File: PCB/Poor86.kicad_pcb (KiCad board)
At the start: 4 copper layers, 100 x 170 mm, 98 parts, among them J1 Bus_ISA_8bit, J2 7-5530843-0, J3 ATX-20, P1 USB_C_Plug_USB2.0, SW3 SW_Push_Dual, SW4 SW_Push_Dual, U1 LFE5U-25F-6BG256C, U10 IS66WVE4M16EBLL-70BLI, U11 CH552T, U2 TLV62569DBV, U3 AM5x86 PQFP208, U4 TLV62569DBV, U5 ESP-12F, U6 TLV62569DBV, U9 IS66WVE4M16EBLL-70BLI

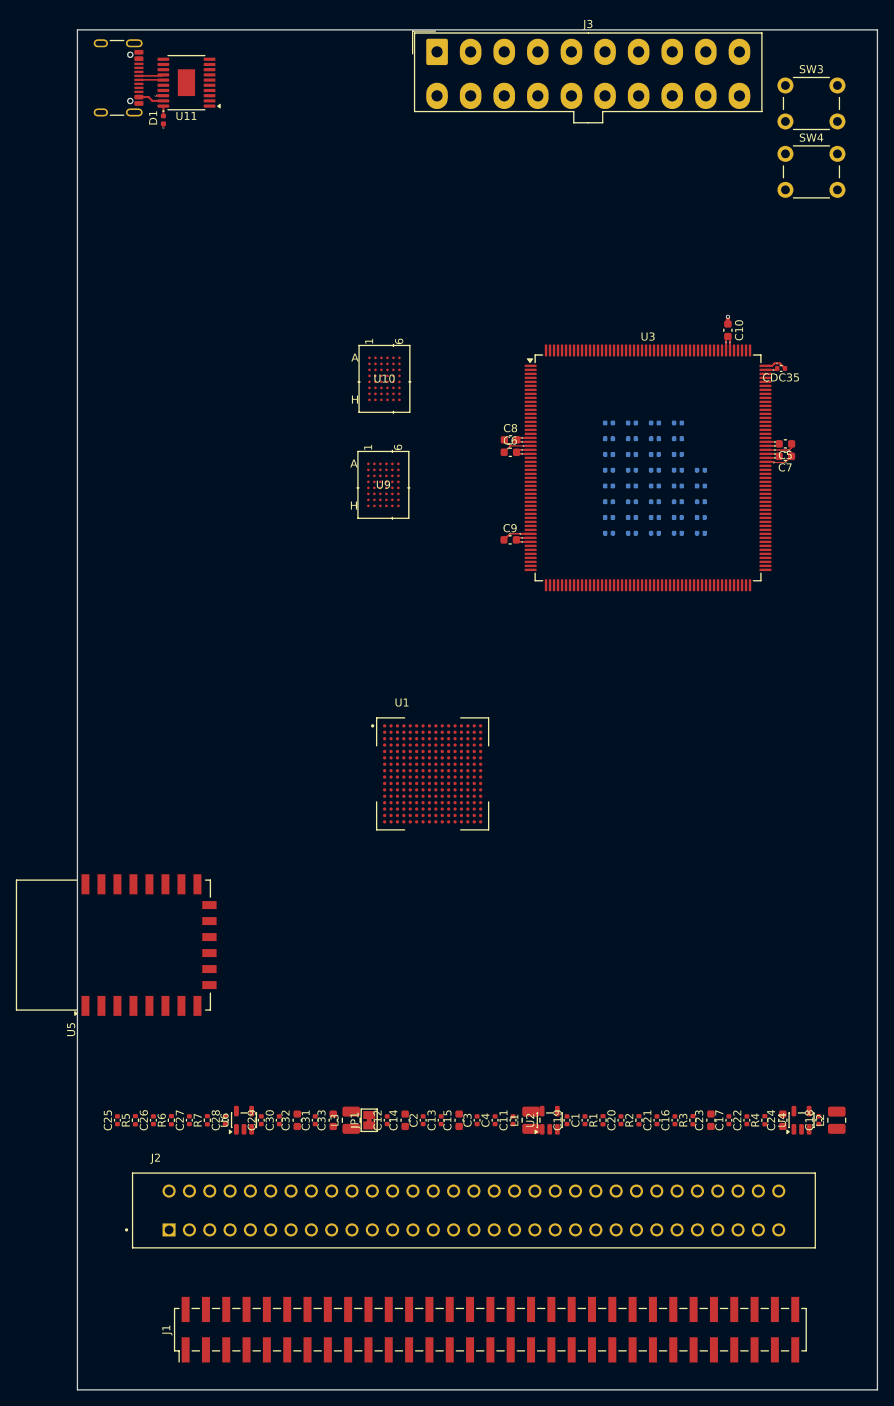
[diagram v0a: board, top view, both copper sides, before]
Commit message: more progress
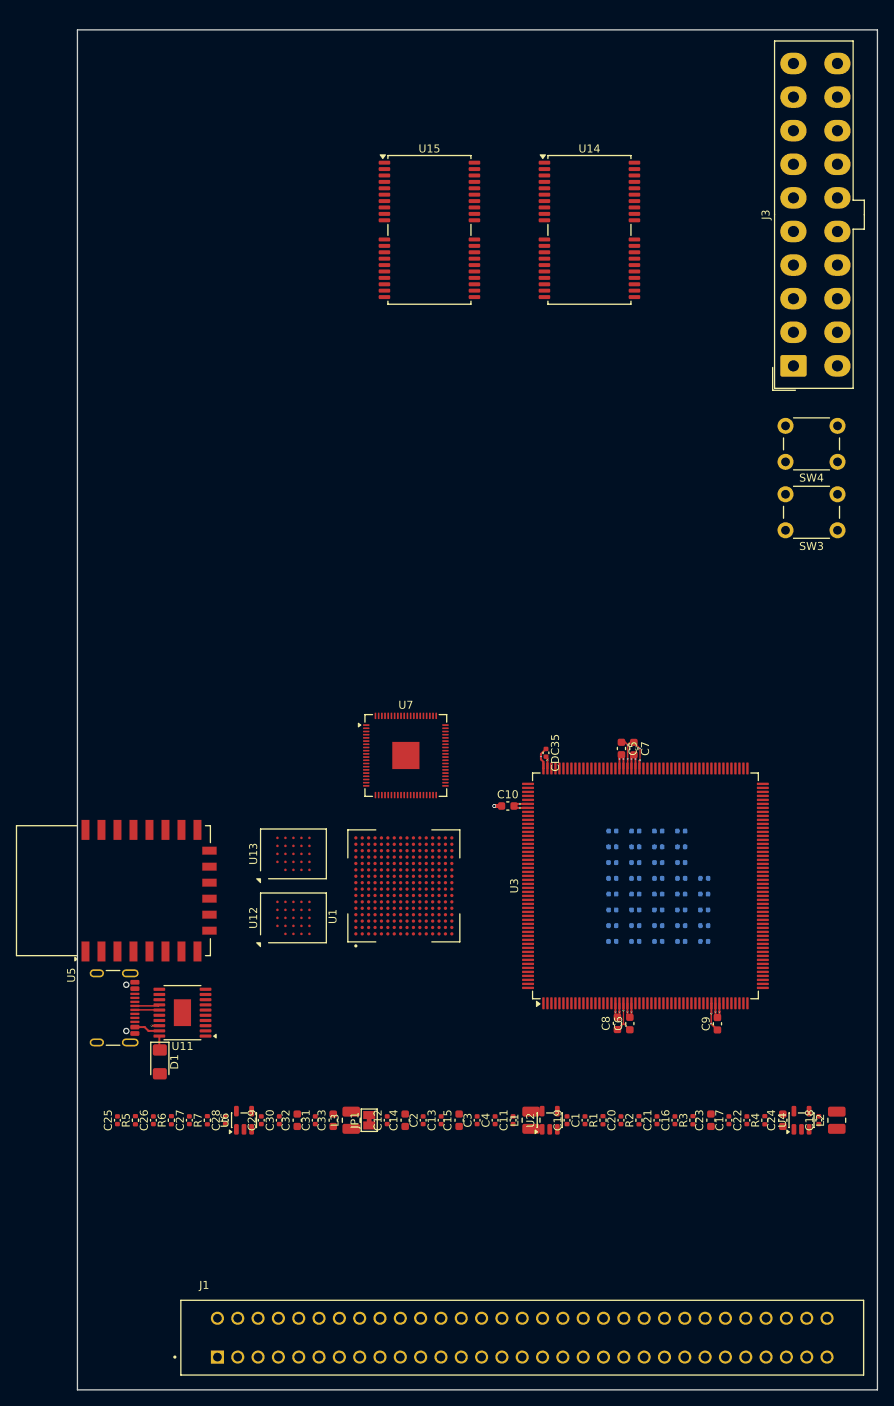
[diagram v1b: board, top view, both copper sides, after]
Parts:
- removed J2: 7-5530843-0, ISA:TE_7-5530843-0
- removed U10, U9: IS66WVE4M16EBLL-70BLI, ISSI:TFBGA48_ISI
- added U12: IS66WVH8M8BLL-100B1LI, Package_BGA:BGA-24_6x8mm_Layout5x5_P1.0mm, F.Cu at (39.0, 123.0)
- added U13: IS66WVH8M8BLL-100B1LI, Package_BGA:BGA-24_6x8mm_Layout5x5_P1.0mm, F.Cu at (39.0, 115.0)
- added U14: KM416x254, Package_SO:TSOP-II-40-44_10.16x18.37mm_P0.8mm, F.Cu at (76.0, 37.0)
- added U15: KM416x254, Package_SO:TSOP-II-40-44_10.16x18.37mm_P0.8mm, F.Cu at (56.0, 37.0)
- added U7: RP2354B, Package_DFN_QFN:QFN-80-1EP_10x10mm_P0.4mm_EP3.4x3.4mm, F.Cu at (53.0, 102.7)
- D1: footprint Diode_SMD:D_0402_1005Metric -> Diode_SMD:D_1206_3216Metric_Pad1.42x1.75mm_HandSolder
- J1: footprint Connector_PinHeader_2.54mm:PinHeader_2x31_P2.54mm_Vertical_SMD -> ISA:TE_7-5530843-0
- moved D1 117.8 mm to (22.3, 141.0)
- moved P1 116.3 mm to (15.5, 134.2)
- moved U11 116.3 mm to (25.1, 134.8)
- moved C8 74.1 mm to (79.5, 136.2), turned to 90 degrees
- moved C6 73.0 mm to (81.0, 136.2), turned to 90 degrees
- moved C9 65.8 mm to (92.0, 136.2), turned to 90 degrees
- moved C10 65.5 mm to (65.8, 109.0), turned to 0 degrees
- moved J3 59.4 mm to (101.5, 54.0), turned to 90 degrees
- moved CDC35 56.3 mm to (70.6, 102.4), turned to -90 degrees
- moved SW3 56.0 mm to (107.0, 74.5), turned to 180 degrees
- moved U3 52.3 mm to (83.0, 119.0), turned to 90 degrees
- moved CDC16 51.0 mm to (81.7, 112.2)
- moved CDC24 51.0 mm to (84.6, 112.2)
- moved CDC32 51.0 mm to (87.5, 112.2)
- moved CDC8 51.0 mm to (78.9, 112.2)
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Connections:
- U1 pad M10: TDO -> Net-(U1H-TDO)
- U3 pad 167: unconnected-(U3B-TMS-Pad167) -> TMS
- U3 pad 168: unconnected-(U3B-TDI-Pad168) -> Net-(U1H-TDO)
- U3 pad 18: unconnected-(U3B-TCK-Pad18) -> TCK
- U3 pad 68: unconnected-(U3B-TDO-Pad68) -> TDO
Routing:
- net Net-(D1-K): track 1.25 -> 1.82 mm
- net +3V3: track 24.6 -> 24.1 mm, vias 14 -> 13
